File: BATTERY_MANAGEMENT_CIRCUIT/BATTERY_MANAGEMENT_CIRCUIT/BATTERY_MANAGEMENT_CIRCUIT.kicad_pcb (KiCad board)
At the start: 2 copper layers, 25.8 x 35.7 mm, 24 parts, among them J1 OUTPUT, J2 BATTERY, J3 Conn_01x02_Socket, J4 Conn_01x02_Socket, J5 UJC-HP-3-SMT-TR, U1 IP5306

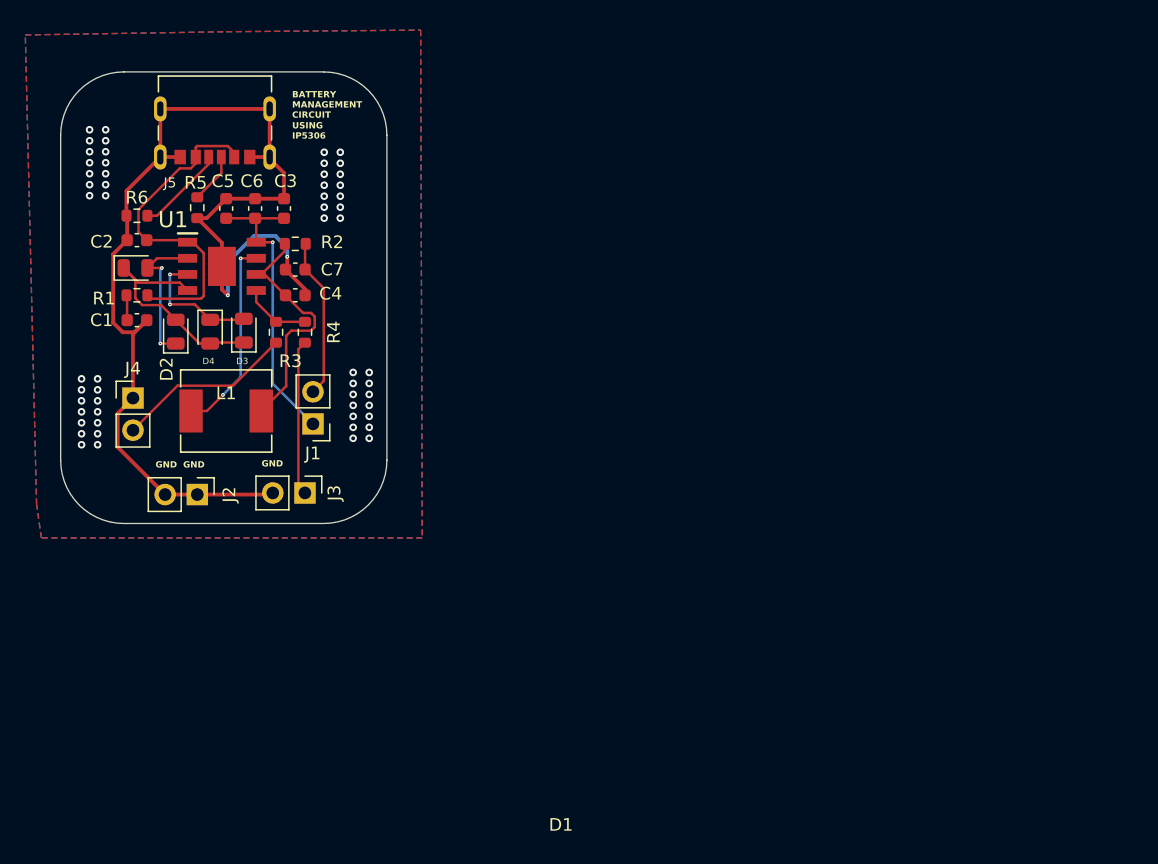
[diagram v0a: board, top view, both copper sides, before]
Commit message: changes and added BMC
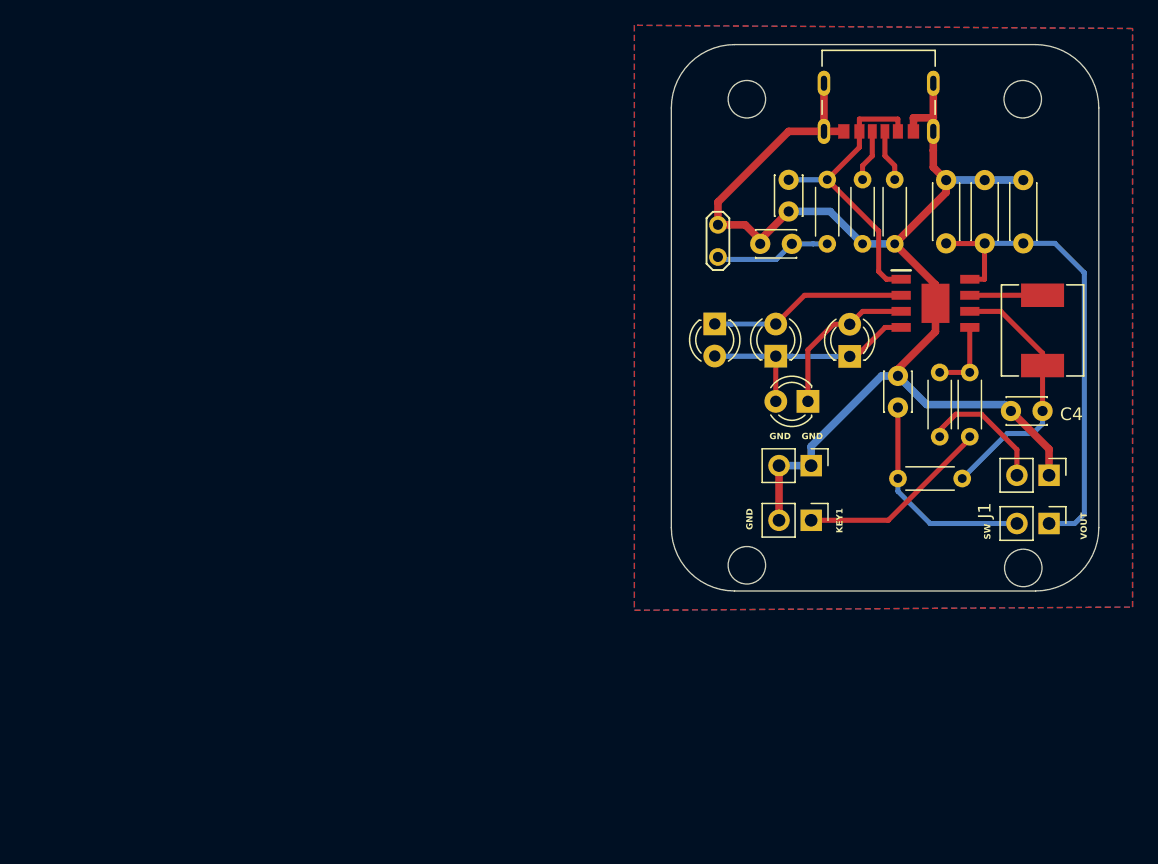
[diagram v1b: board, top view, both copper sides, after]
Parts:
- added J6: TP1, TestPoint:TestPoint_2Pads_Pitch2.54mm_Drill0.8mm, F.Cu at (115.3, 56.9)
- C1, C2, C4, C7: footprint Capacitor_SMD:C_0603_1608Metric -> Capacitor_THT:C_Disc_D3.0mm_W2.0mm_P2.50mm
- C3, C5, C6: footprint Capacitor_SMD:C_0603_1608Metric -> Capacitor_THT:C_Disc_D4.3mm_W1.9mm_P5.00mm
- D1, D2, D3, D4: footprint LED_SMD:LED_0805_2012Metric -> LED_THT:LED_D3.0mm
- R1, R2, R3, R4, R5, R6: footprint Resistor_SMD:R_0603_1608Metric -> Resistor_THT:R_Axial_DIN0204_L3.6mm_D1.6mm_P5.08mm_Horizontal
- moved J4 72.7 mm to (141.5, 76.7), turned to -90 degrees
- moved L1 64.8 mm to (141.0, 65.3), turned to -90 degrees
- moved C5 63.1 mm to (139.4, 58.4)
- moved C4 59.8 mm to (141.0, 71.6), turned to 180 degrees
- moved J1 58.7 mm to (141.5, 80.5), turned to -90 degrees
- moved C6 57.7 mm to (136.4, 58.4)
- moved R6 57.4 mm to (126.7, 58.4), turned to 90 degrees
- moved U1 56.5 mm to (132.5, 63.1)
- moved R2 55.9 mm to (134.6, 77.0), turned to 180 degrees
- moved R1 55.3 mm to (124.0, 53.3), turned to -90 degrees
- moved R5 55.2 mm to (129.3, 58.4)
- moved R4 53.2 mm to (135.2, 73.7)
- moved R3 53.1 mm to (132.8, 73.7)
- moved J5 52.5 mm to (128.0, 49.5)
- moved C3 52.4 mm to (133.3, 58.4)
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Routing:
- net /VOUT: track 23.5 -> 38.0 mm, vias 1 -> 0
- net GND: track 94.0 -> 105.1 mm, vias 58 -> 0
- net Net-(U1-SW): track 15.7 -> 5.75 mm, vias 2 -> 0
- net Net-(J6-Pin_2): track 1.99 -> 9.23 mm
- net Net-(J1-Pin_2): track 12.7 -> 17.1 mm
- net Net-(J4-Pin_2): track 14.2 -> 10.3 mm
- net /LED1: track 11.9 -> 15.7 mm, vias 2 -> 0
- net Net-(J3-Pin_1): track 12.3 -> 15.4 mm
- net /CC2: track 7.09 -> 4.12 mm
- net VCC: track 26.6 -> 23.9 mm
- net /LED2: track 10.1 -> 12.7 mm, vias 2 -> 0
- net Net-(U1-BAT): track 19.7 -> 20.8 mm
- net /LED3: track 18.7 -> 19.3 mm
- net Net-(U1-KEY): track 5.41 -> 5.93 mm
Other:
- board size 25.8 x 35.7 mm -> 33.8 x 43.2 mm
- board text added: "KEY1"
- board text added: "SW"
- board text added: "VOUT"
- board text removed: "BATTERY MANAGEMENT CIRCUIT"
- board text removed: "GND GND"
- board text removed: "USING IP5306"
